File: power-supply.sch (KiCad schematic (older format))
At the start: 32 parts, among them J18 Conn_01x02_Male, U11 BA33BC0FP-E2, U13 LM2990SX-5.0, U14 BA50BC0FP-E2, U15 10M08SC

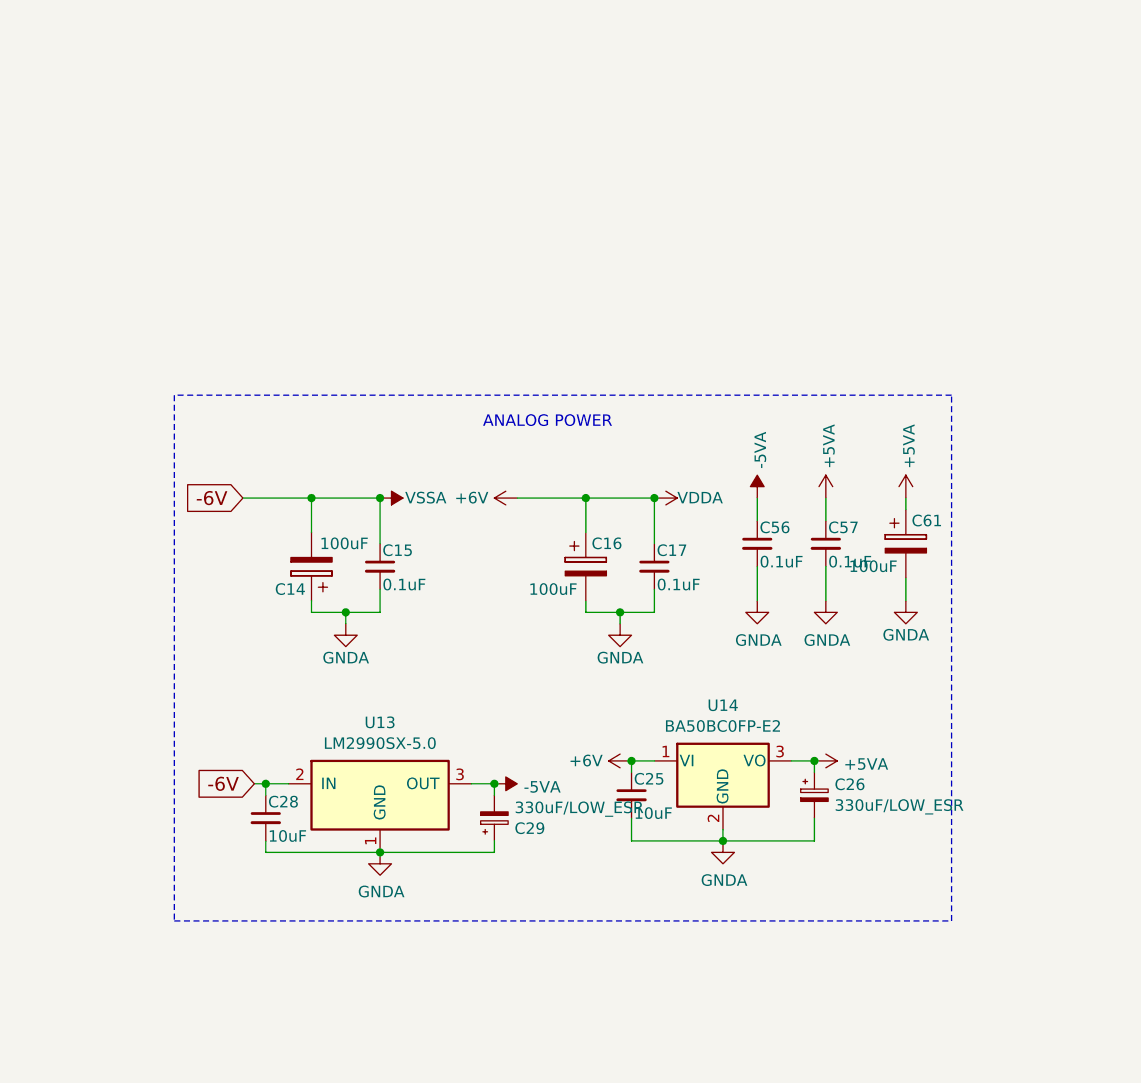
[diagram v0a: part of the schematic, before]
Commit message: Rev. E
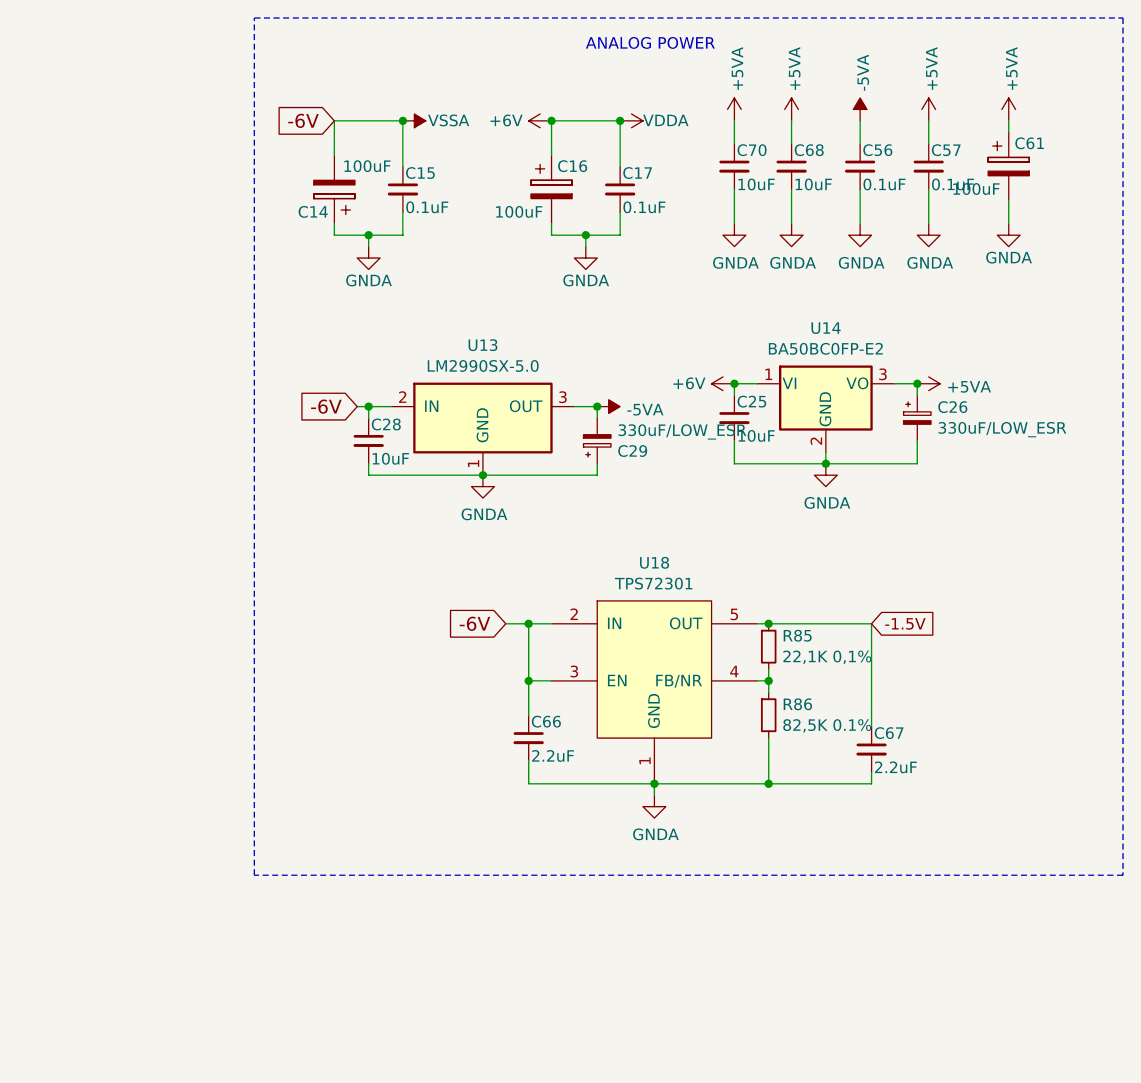
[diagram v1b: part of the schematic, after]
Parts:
- added C66, C67: 2.2uF, Capacitor_SMD:C_0805_2012Metric_Pad1.18x1.45mm_HandSolder, symbol bkm-68x-simple-rescue:C_Small
- added C68, C70: 10uF, Capacitor_SMD:C_0805_2012Metric_Pad1.18x1.45mm_HandSolder, symbol bkm-68x-simple-rescue:C_Small
- added R85: 22,1K 0,1%, Resistor_SMD:R_0805_2012Metric_Pad1.20x1.40mm_HandSolder, symbol Device:R_Small
- added R86: 82,5K 0.1%, Resistor_SMD:R_0805_2012Metric_Pad1.20x1.40mm_HandSolder, symbol Device:R_Small
- added U18: TPS72301, Package_TO_SOT_SMD:SOT-23-5, symbol tps723xx:TPS723xx
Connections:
- net +5VA: now also C68.1, C70.1
- net GNDA: now also C66.2, C67.2, C68.2, C70.2, R86.2, U18.1 (GND)
- net VSSA: now also C66.1, U18.2 (IN), U18.3 (EN)
- new net: R85.2, R86.1, U18.4 (FB/NR)
- new net -1.5V: C67.1, R85.1, U18.5 (OUT)
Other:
- moved on the sheet: C14, C15, C16, C17, C25, C26, C28, C29, C56, C57, C61, U13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
